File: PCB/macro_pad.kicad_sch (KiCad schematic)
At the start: 56 parts, among them J1 OLED, J2 SWD, SW1 SW_Push_45deg, SW10 SW_Push_45deg, SW11 SW_Push_45deg, SW12 SW_Push_45deg, SW13 SW_Push_45deg, SW14 SW_Push_45deg, SW15 SW_Push_45deg, SW16 SW_Push_45deg, SW17 RotaryEncoder_Switch, SW18 RotaryEncoder_Switch, SW2 SW_Push_45deg, SW3 SW_Push_45deg, SW4 SW_Push_45deg, SW5 SW_Push_45deg, SW6 SW_Push_45deg, SW7 SW_Push_45deg, SW8 SW_Push_45deg, SW9 SW_Push_45deg

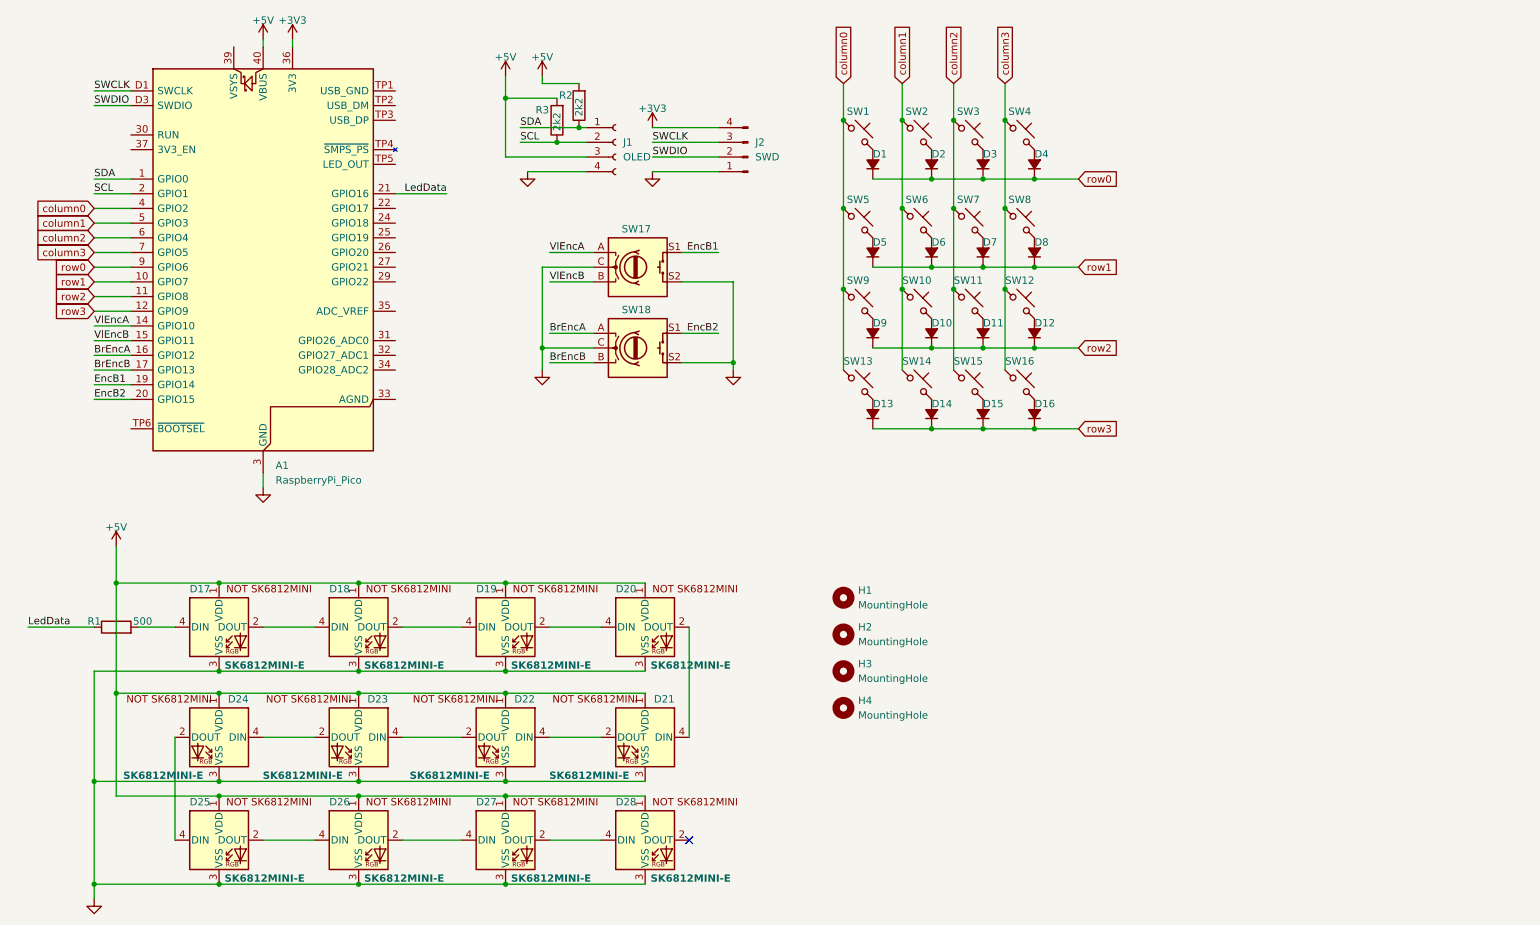
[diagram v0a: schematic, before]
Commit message: Followed guidelines on schem
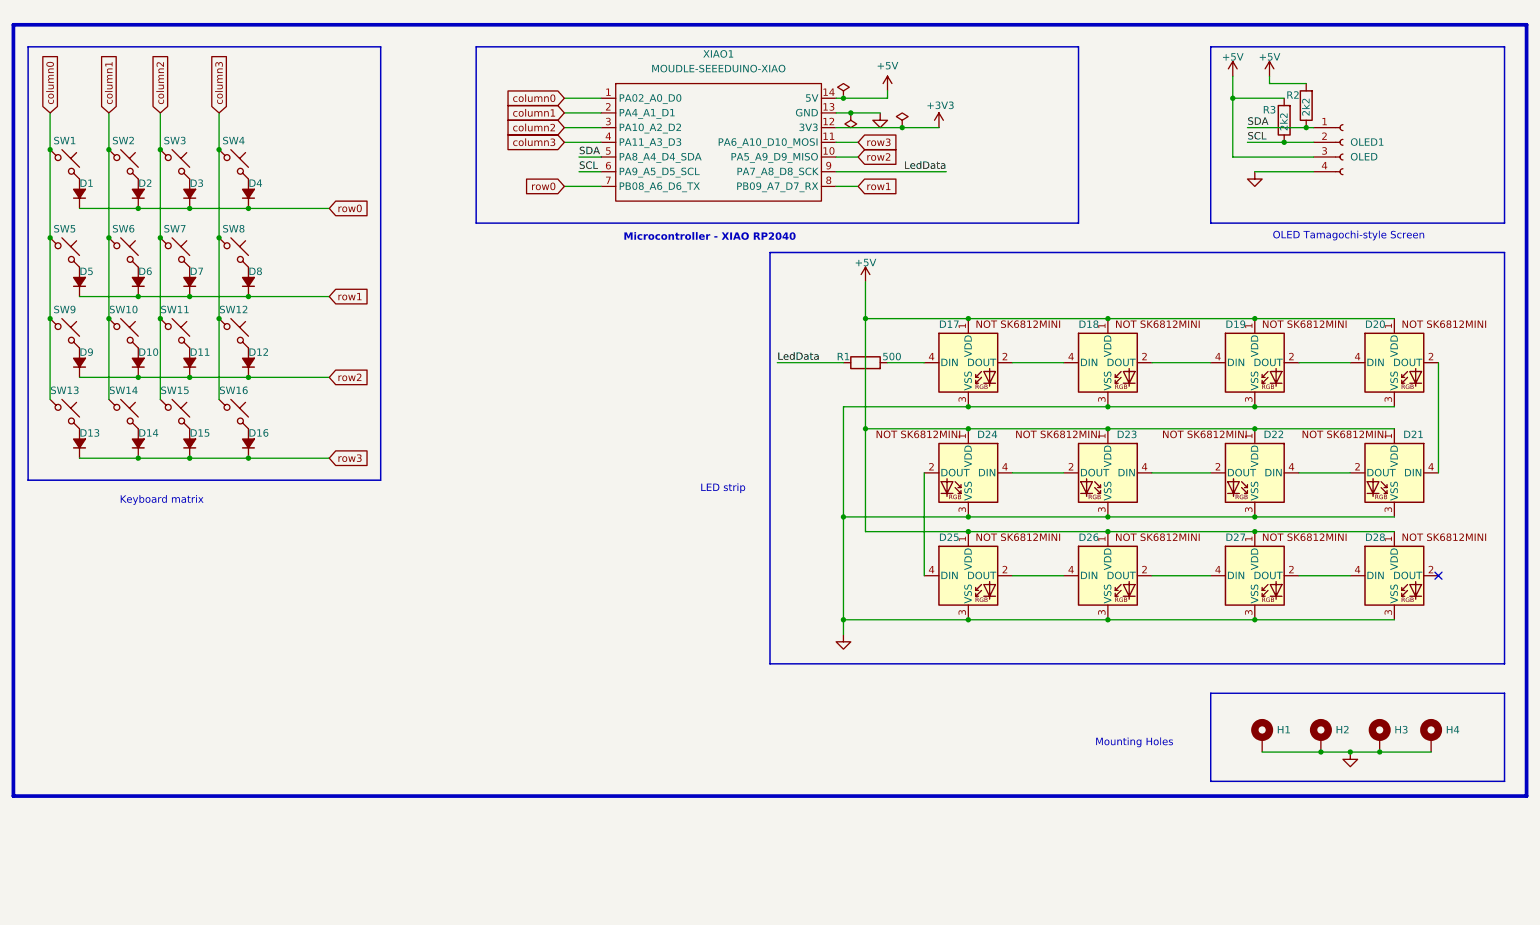
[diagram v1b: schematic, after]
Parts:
- removed A1: RaspberryPi_Pico, Module:RaspberryPi_Pico_SMD, symbol MCU_Module:RaspberryPi_Pico_Extensive
- removed H1, H2, H3, H4: MountingHole, MountingHole:MountingHole_3.2mm_M3, symbol Mechanical:MountingHole
- removed J2: SWD, Connector_PinHeader_2.54mm:PinHeader_1x04_P2.54mm_Vertical, symbol Connector:Conn_01x04_Pin
- removed SW17, SW18: RotaryEncoder_Switch, RotaryEncoder_Alps_EC11E-Switch_Vertical_H20mm:RotaryEncoder_Alps_EC11E-Switch_Vertical_H20mm, symbol Device:RotaryEncoder_Switch
- added H1, H2, H3, H4: MountingHole_Pad, MountingHole:MountingHole_3.2mm_M3_ISO7380_Pad, symbol Mechanical:MountingHole_Pad
- added XIAO1: MOUDLE-SEEEDUINO-XIAO, XIAO_RP2040:XIAO_RP2040, symbol XIAO_RP2040:MOUDLE-SEEEDUINO-XIAO
- renumbered J1 to OLED1
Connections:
- net +3V3: now also XIAO1.12 (3V3)
- net +5V: now also XIAO1.14 (5V)
- net GND: now also H1.1, H2.1, H3.1, H4.1, XIAO1.13 (GND)
- net LedData: now also XIAO1.9 (PA7_A8_D8_SCK)
- net SCL: now also XIAO1.6 (PA9_A5_D5_SCL)
- net SDA: now also XIAO1.5 (PA8_A4_D4_SDA)
- net column0: now also XIAO1.1 (PA02_A0_D0)
- net column1: now also XIAO1.2 (PA4_A1_D1)
- net column2: now also XIAO1.3 (PA10_A2_D2)
- net column3: now also XIAO1.4 (PA11_A3_D3)
- net row0: now also XIAO1.7 (PB08_A6_D6_TX)
- net row1: now also XIAO1.8 (PB09_A7_D7_RX)
- net row2: now also XIAO1.10 (PA5_A9_D9_MISO)
- net row3: now also XIAO1.11 (PA6_A10_D10_MOSI)
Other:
- note added: "Keyboard matrix"
- note added: "LED strip"
- note added: "Microcontroller - XIAO RP2040"
- note added: "Mounting Holes"
- note added: "OLED Tamagochi-style Screen"
- moved on the sheet: D1, D17, D18, D19, D2, D20, D21, D22, D23, D24, D25, D3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
